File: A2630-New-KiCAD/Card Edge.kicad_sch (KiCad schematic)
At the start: 35 parts, among them CN700 Amiga-2000-CPU-Slot, J301 Jumper_NO_Small, J302 Jumper_NO_Small, J303 Jumper_NO_Small, J304 Jumper_NO_Small, J305 Jumper_NO_Small, U300 74HCT05, U307 74HCT04, U700 74HCT174, U701 74FCT646, U702 74FCT646, U703 74HCT245, U704 74HCT245, U705 74HCT245, U706 74HCT245, U707 74HCT245

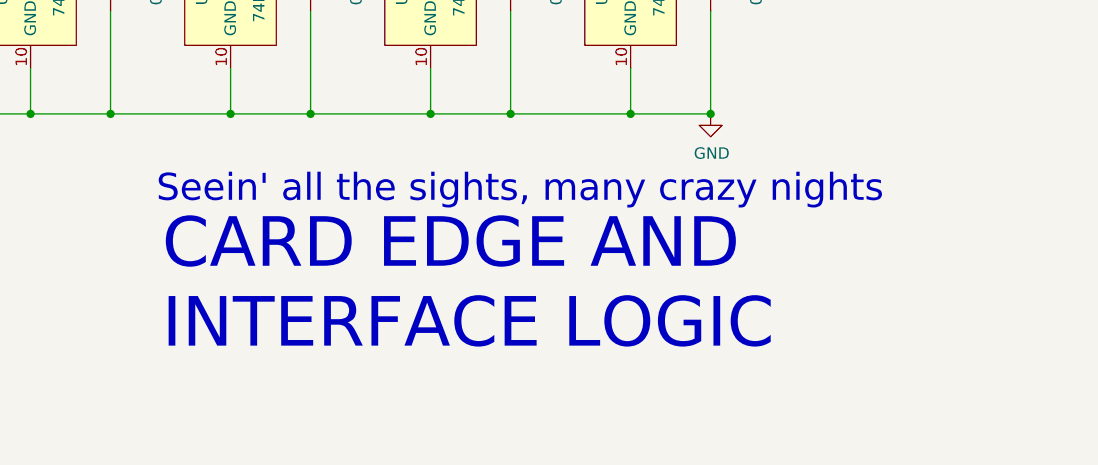
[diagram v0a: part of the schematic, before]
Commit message: Add files via upload
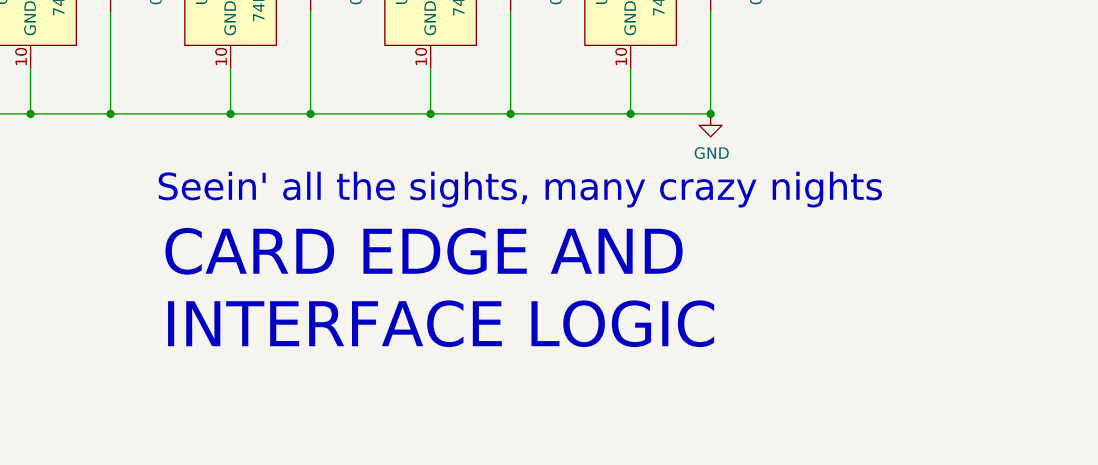
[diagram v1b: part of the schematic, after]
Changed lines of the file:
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@@
   )
   (text "CARD EDGE AND\nINTERFACE LOGIC" (at 313.055 250.825 0)
-    (effects (font (size 5.5118 5.5118)) (justify left bottom))
+    (effects (font (size 5 5)) (justify left bottom))
   )
   (label "AA23" (at 265.43 48.895 0)
